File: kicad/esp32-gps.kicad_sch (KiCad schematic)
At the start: 30 parts, among them J1 Conn_01x07_Socket, Q1 BCW66G, Q2 BCW66G, SW1 RESET, SW2 BOOT, U1 ESP32-PICO-V3, U2 CH340C

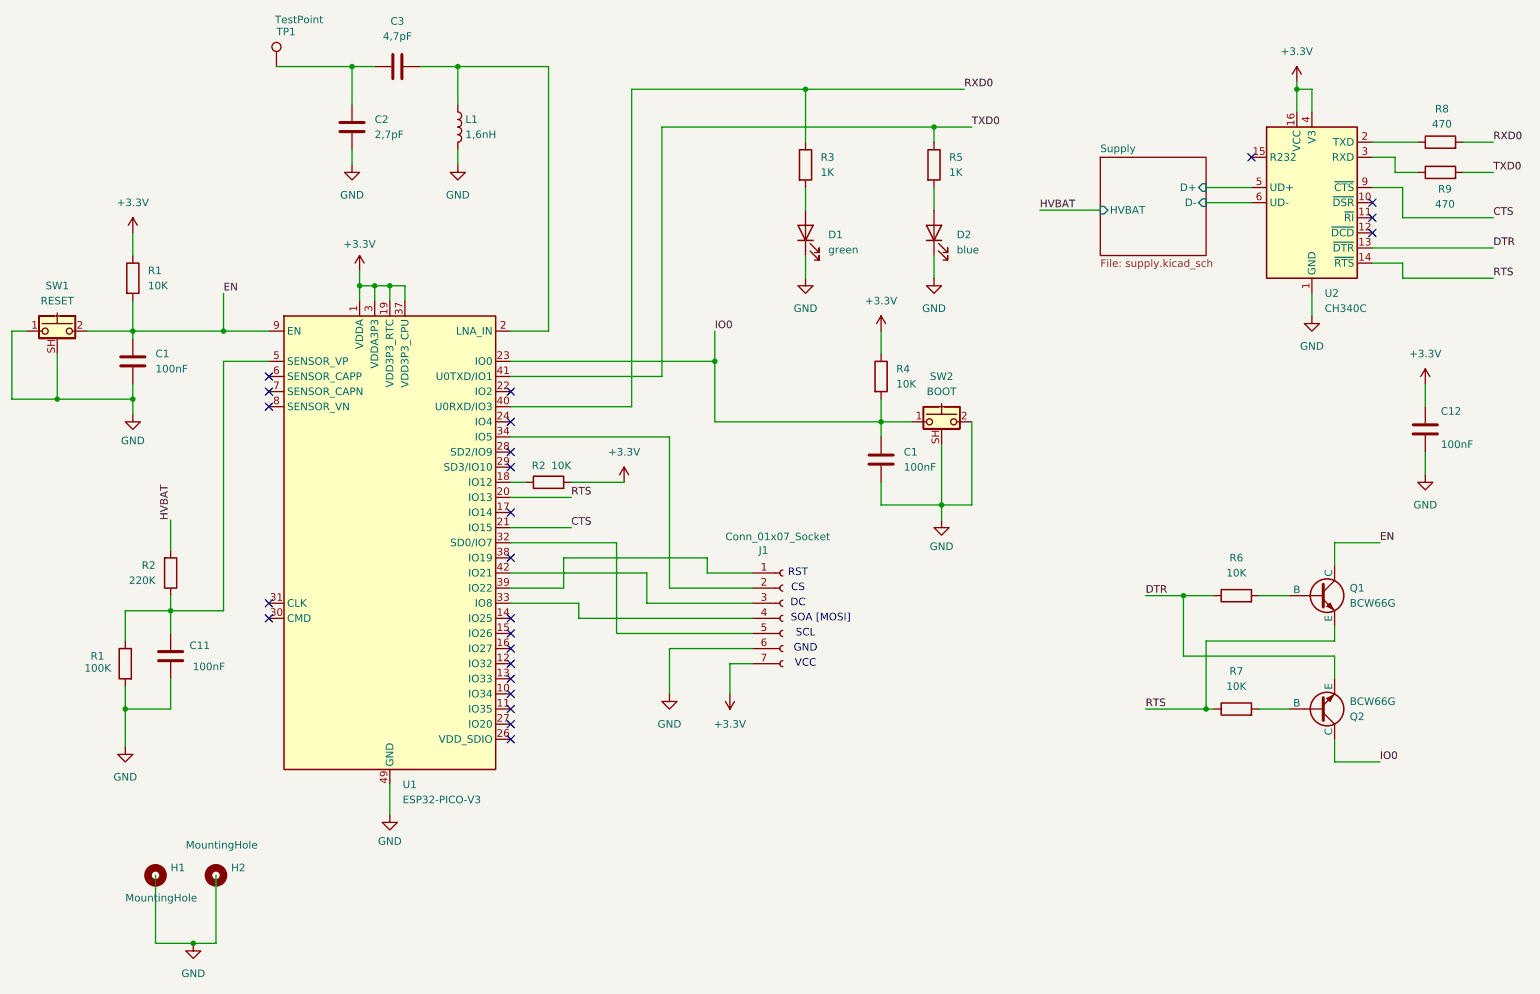
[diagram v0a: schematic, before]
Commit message: init
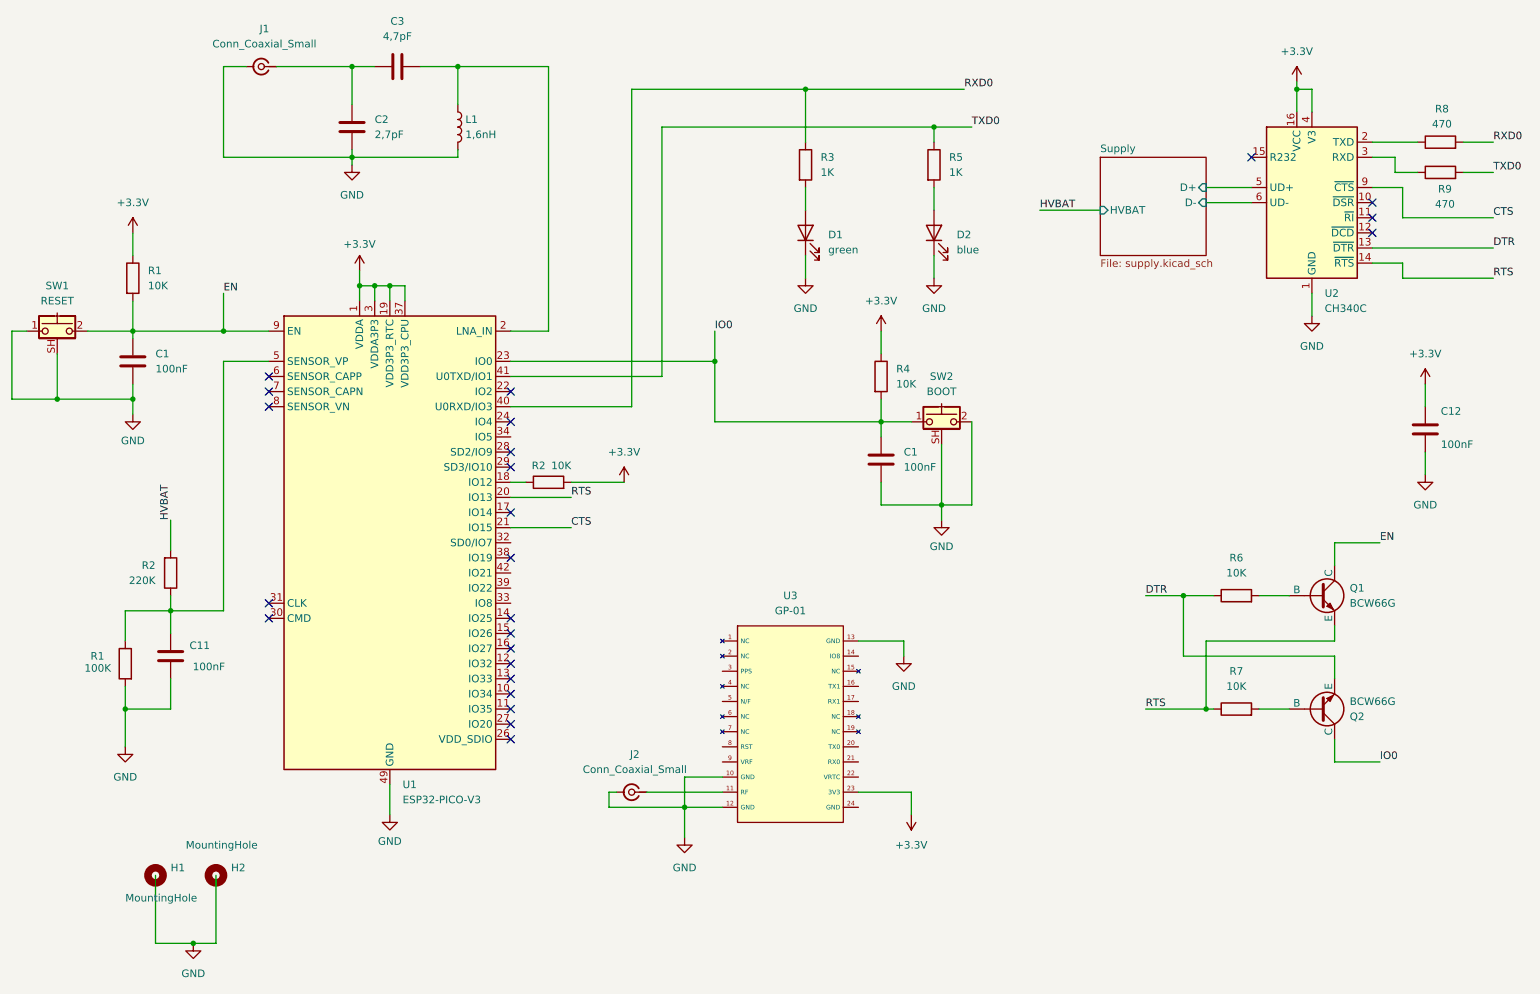
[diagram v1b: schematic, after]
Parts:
- removed J1: Conn_01x07_Socket, Connector_PinSocket_2.54mm:PinSocket_1x07_P2.54mm_Vertical, symbol Connector:Conn_01x07_Socket
- removed TP1: TestPoint, TestPoint:TestPoint_Pad_3.0x3.0mm, symbol Connector:TestPoint
- added J1, J2: Conn_Coaxial_Small, Connector_Coaxial:U.FL_Molex_MCRF_73412-0110_Vertical, symbol Connector:Conn_Coaxial_Small
- added U3: GP-01, PCM_yvolodym:GP-01, symbol PCM_yvolodym:GP-01
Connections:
- net +3.3V: now also U3.23 (3V3)
- net GND: now also J1.2 (Ext), J2.2 (Ext), U3.10 (GND), U3.12 (GND), U3.13 (GND)
- net at C2.1, C3.1: now also J1.1 (In)
- new net: J2.1 (In), U3.11 (RF)
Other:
- note removed: "CS"
- note removed: "DC"
- note removed: "GND"
- note removed: "RST"
- note removed: "SCL"
- note removed: "SOA [MOSI]"
- note removed: "VCC"
